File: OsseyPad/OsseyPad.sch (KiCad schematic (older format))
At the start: 90 parts, among them SW1 Rotary_Encoder_Switch, SW2 Rotary_Encoder_Switch, SW3 SW_Push, U1 ATmega32U4-MU, Y1 16MHz

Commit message: Updated the pcb.
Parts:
- removed C6, C7: 22pF, Capacitor_SMD:C_0603_1608Metric, symbol Device:C
- removed D32: PRTR5V0U2X, Package_TO_SOT_SMD:SOT-143, symbol Power_Protection:PRTR5V0U2X
- removed FB2: 50 @ 100 MHz, Inductor_SMD:L_0805_2012Metric, symbol Device:Ferrite_Bead
- removed R1, R2: 5.1k, Resistor_SMD:R_0603_1608Metric, symbol Device:R
- removed SW1: Rotary_Encoder_Switch, symbol Device:Rotary_Encoder_Switch
- removed USB1: HRO-TYPE-C-31-M-12, symbol Type-C:HRO-TYPE-C-31-M-12
- added C10, C9: 100n, Capacitor_SMD:C_0603_1608Metric, symbol Device:C_Small
- added C6, C7: 15pF, Capacitor_SMD:C_0603_1608Metric, symbol Device:C_Small
- added J1: USB_C_Receptacle_USB2.0, josh-connectors:USB_C_U262-161N-4BVC11, symbol Connector:USB_C_Receptacle_USB2.0
- added R10, R11: 5K1, Resistor_SMD:R_0603_1608Metric, symbol Device:R_Small
- added R5, R6, R7, R8, R9: 10K, Resistor_SMD:R_0603_1608Metric, symbol Device:R_Small
- added U1: USBLC6-2SC6, Package_TO_SOT_SMD:SOT-23-6, symbol Power_Protection:USBLC6-2SC6
- SW1: renamed from SW2; footprint (none) -> Rotary_Encoder:RotaryEncoder_Alps_EC11E-Switch_Vertical_H20mm_CircularMountingHoles
- SW2: renamed from SW3; footprint Button_Switch_SMD:SW_Push_1P1T_NO_6x6mm_H9.5mm -> Button_Switch_THT:SW_PUSH_6mm_H5mm
- renumbered D9 to D10, D10 to D11, D11 to D12, D12 to D13, D13 to D14, D14 to D15, D15 to D16, D16 to D17, D17 to D18, D18 to D19, D19 to D20, D20 to D21, D21 to D22, D22 to D23, D23 to D24, D24 to D25, D25 to D26, D26 to D27, D27 to D28, D28 to D29, D29 to D30, D30 to D31, D31 to D32, D5 to D6, D6 to D7, D7 to D8, D8 to D9, R5 to R1, R3 to R2, R4 to R3, R6 to R4, U1 to U2
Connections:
- net labels added: ENC_1_A, ENC_1_B, ENC_1_SW, RESET, USB_CONN_D+, USB_CONN_D-, VCC, XTAL1, XTAL2
- net labels removed: VBUS
- wire segments 251 -> 266
- no-connect marks 2 -> 14
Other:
- moved on the sheet: C1, C2, C3, C4, C5, C8, H1, H2, H3, H4, R1, R2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

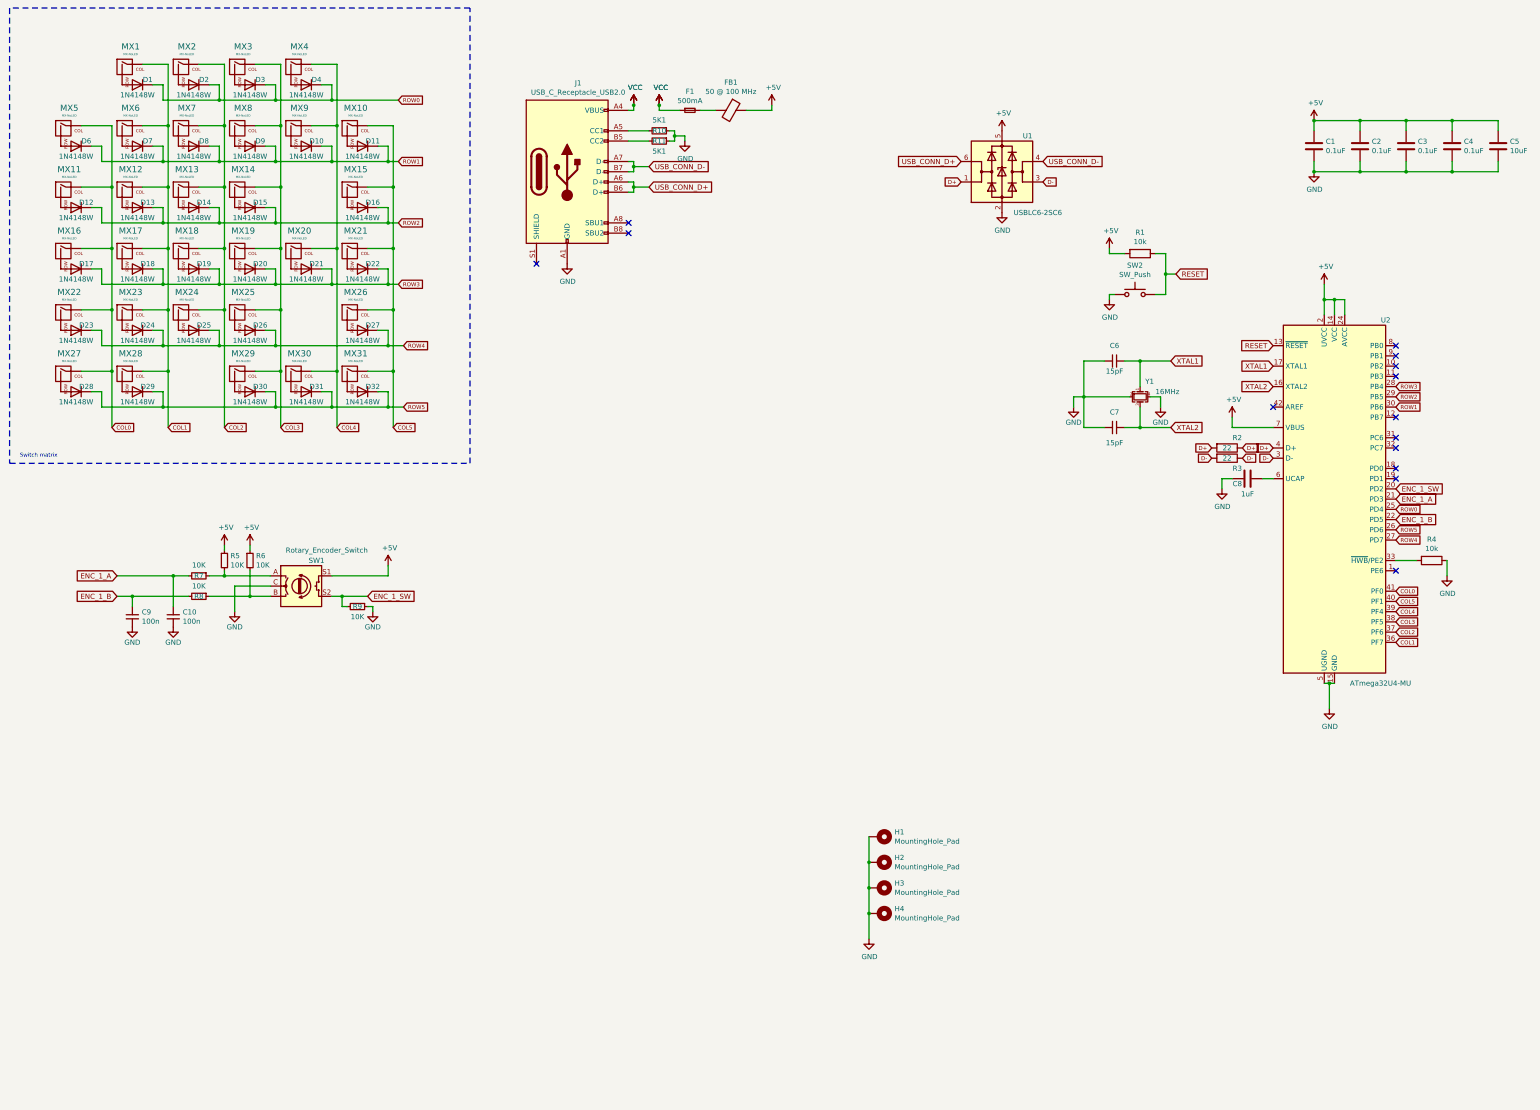
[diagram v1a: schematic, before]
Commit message: Updatet the pcb and added first versio off the firmware.
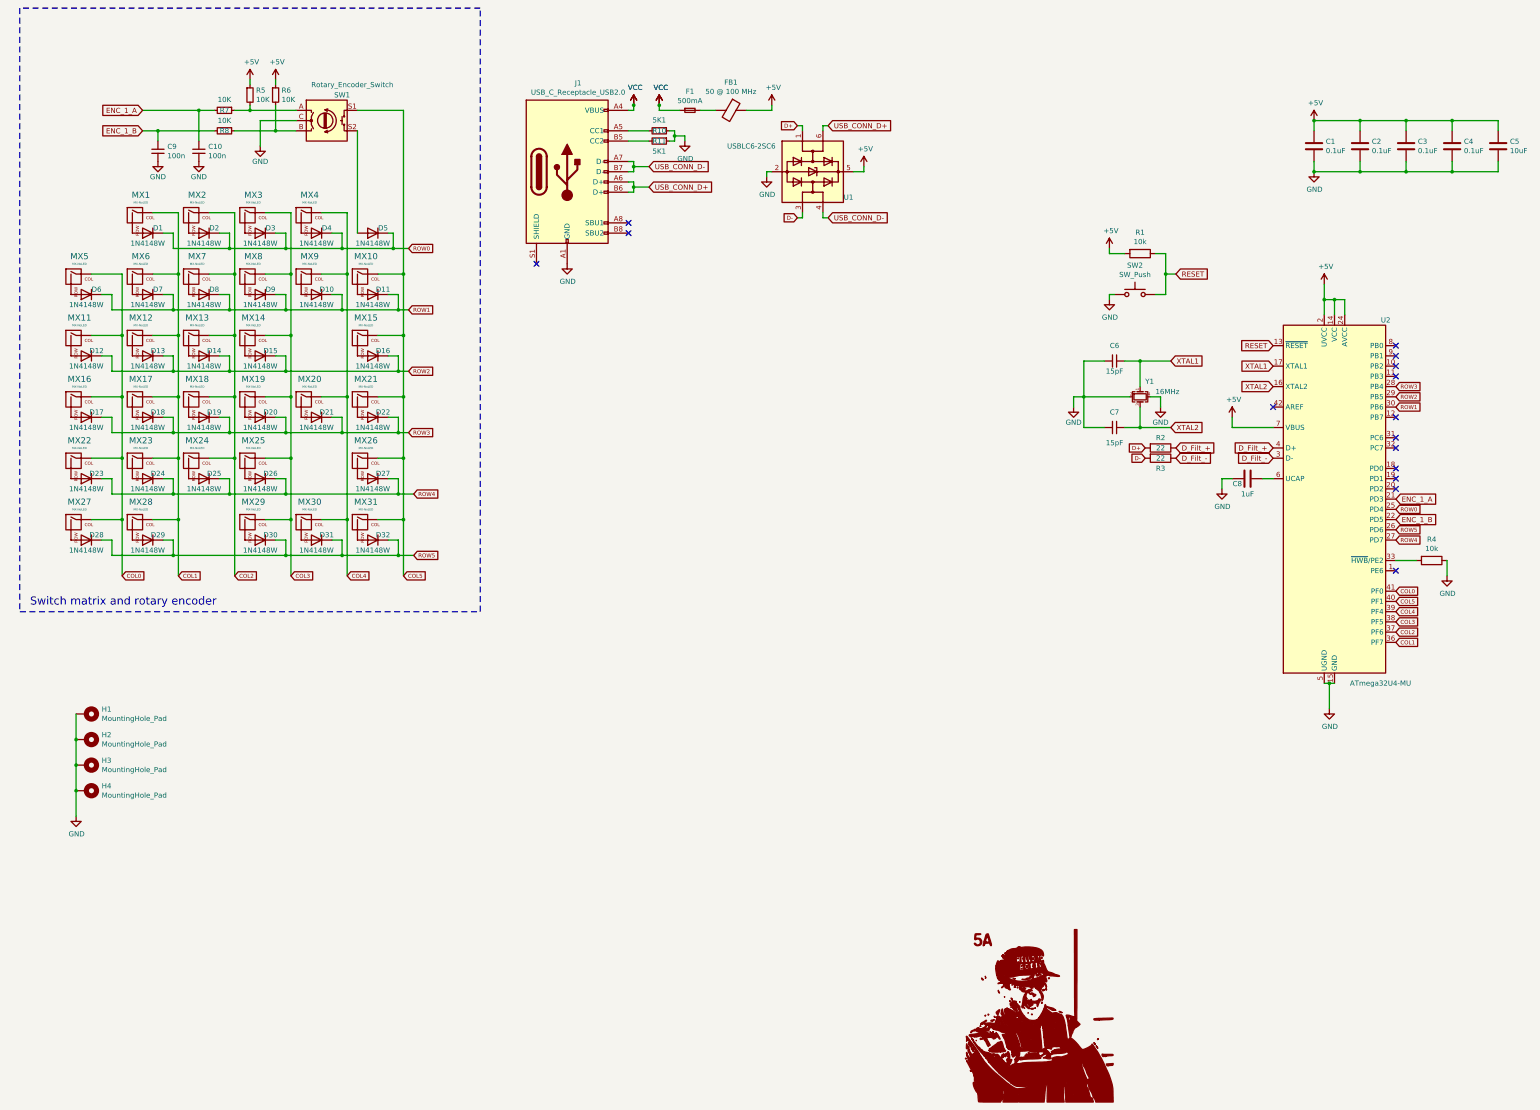
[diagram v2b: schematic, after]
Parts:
- removed R9: 10K, Resistor_SMD:R_0603_1608Metric, symbol Device:R_Small
- added D5: 1N4148W, Diode_SMD:D_SOD-123, symbol Diode:1N4148
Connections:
- net +5V: no longer SW1.S1
- net COL5: now also SW1.S1
- net D+: no longer R2.1, U2.4 (D+)
- net D-: no longer R3.1, U2.3 (D-)
- net ROW0: now also D5.1 (K)
- net ENC_1_SW: no longer names the net of SW1.S2
- net ENC_1_SW: now also D5.2 (A); no longer U2.20 (PD2)
- new net D_Filt_+: R2.1, U2.4 (D+)
- new net D_Filt_-: R3.1, U2.3 (D-)
- no-connect marks 14 -> 15
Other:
- note added: "Switch matrix and rotary encoder"
- note removed: "Switch matrix\n"
- moved on the sheet: C10, C9, D1, D10, D11, D12, D13, D14, D15, D16, D17, D18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
